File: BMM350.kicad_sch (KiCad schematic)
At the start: 2 parts, among them U8 BMM350

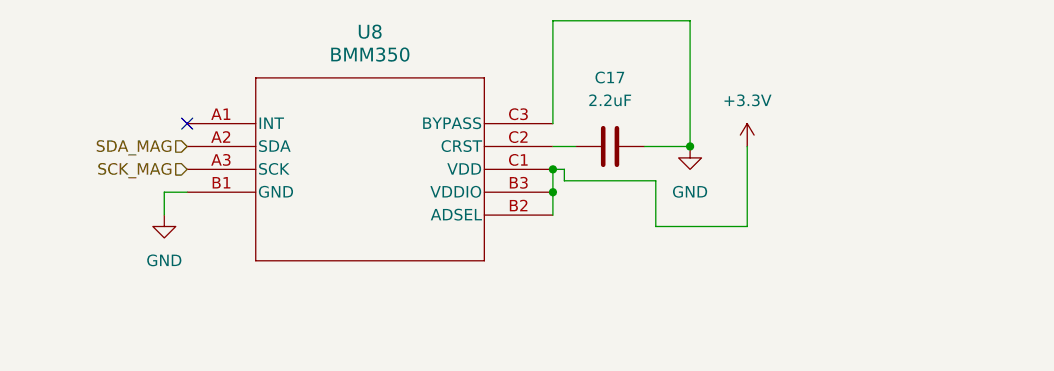
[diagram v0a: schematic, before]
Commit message: branches
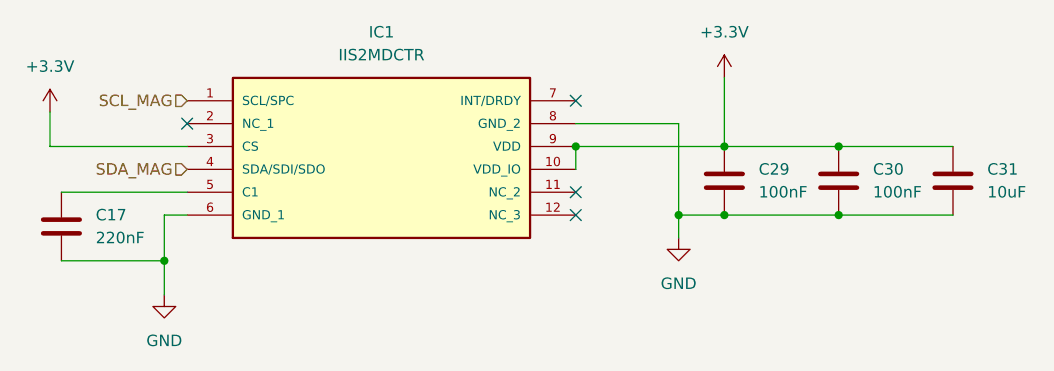
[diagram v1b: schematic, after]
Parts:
- removed U8: BMM350, BGA9_BMM350_BOS, symbol BMM350:BMM350
- added C29, C30: 100nF, Capacitor_SMD:C_0402_1005Metric, symbol Device:C
- added C31: 10uF, Capacitor_SMD:C_0201_0603Metric, symbol Device:C
- added IC1: IIS2MDCTR, IIS2MDCTR:IIS2MDCTR, symbol IIS2MDCTR:IIS2MDCTR
- C17: value 2.2uF -> 220nF
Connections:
- net +3.3V: now also C29.1, C30.1, C31.1, IC1.10 (VDD_IO), IC1.3 (CS), IC1.9 (VDD)
- net GND: now also C29.2, C30.2, C31.2, IC1.6 (GND_1), IC1.8 (GND_2)
- net SDA_MAG: now also IC1.4 (SDA/SDI/SDO)
- net at C17.1: now also IC1.5 (C1)
- new net SCL_MAG: IC1.1 (SCL/SPC)
- no-connect marks 1 -> 4
